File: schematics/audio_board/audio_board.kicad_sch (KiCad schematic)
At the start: 42 parts, among them J1 servo ctrl, J2 Speaker, J3 I2S, Q1 PMOS, Q2 NPN, U1 TPS613222ADBV, U2 MAX98357A, U3 TPS613222ADBV, U4 TPS613222ADBV, U8 MCP73812

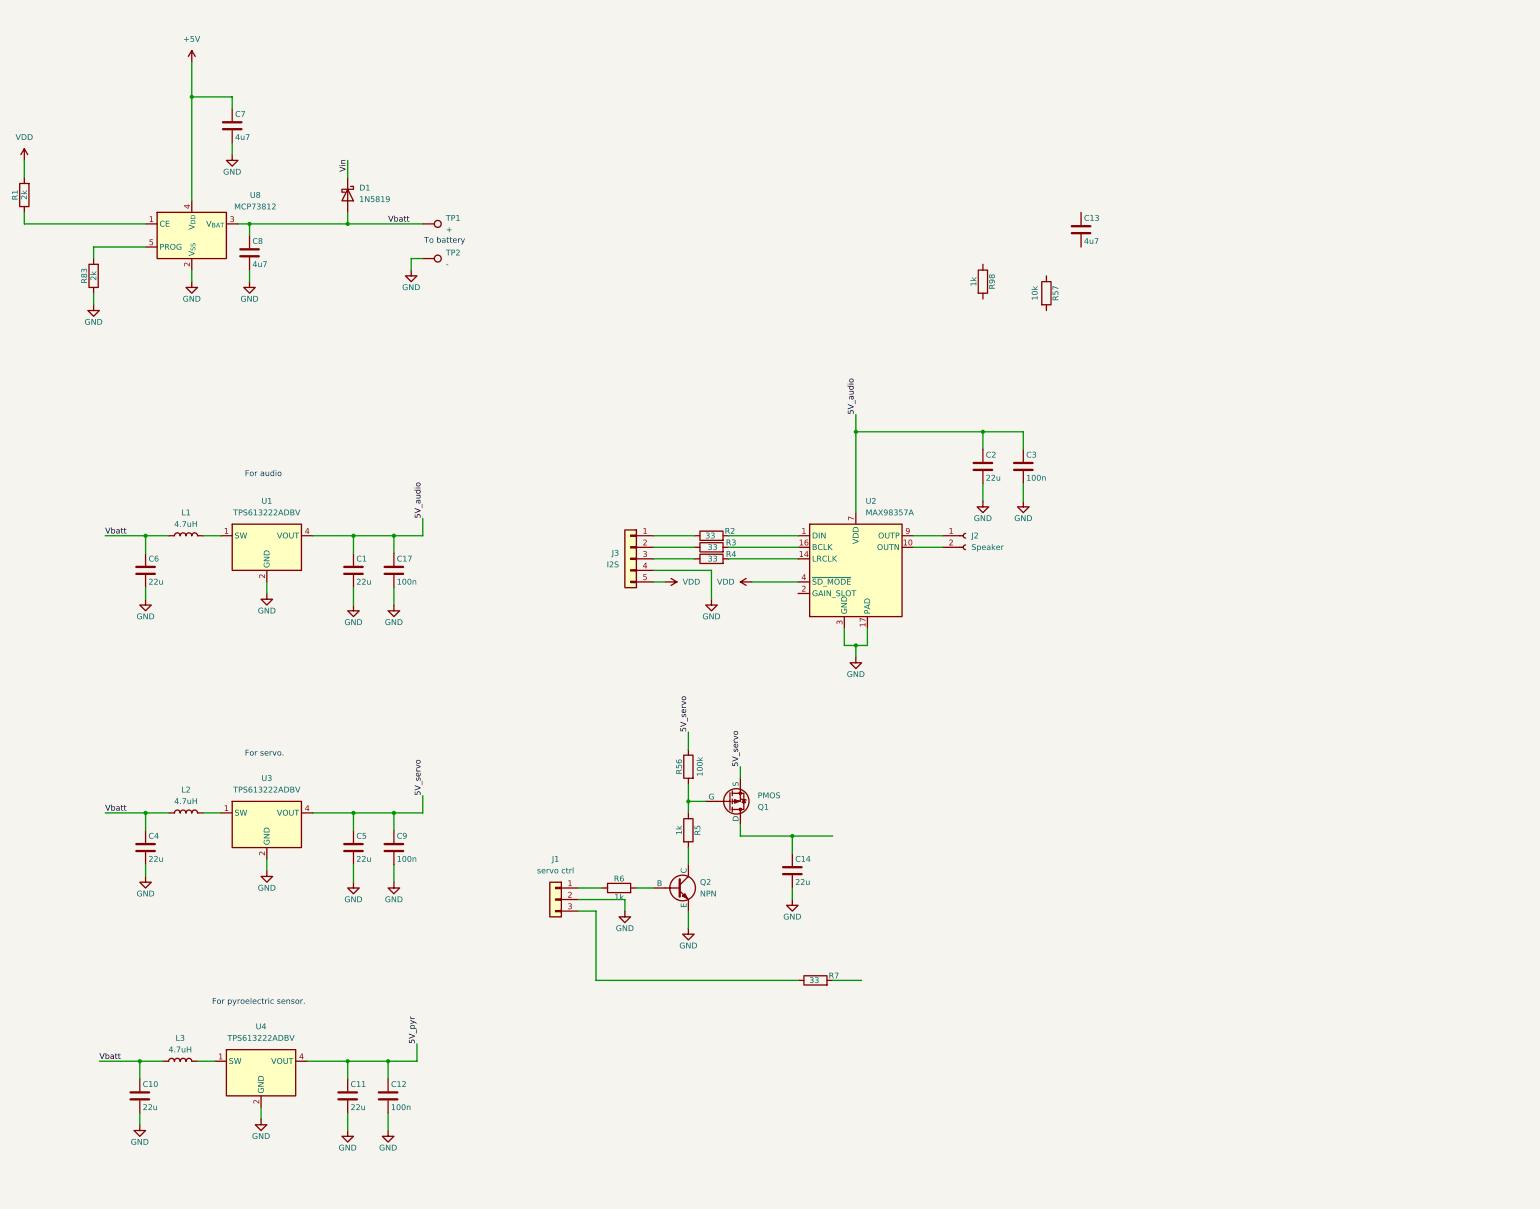
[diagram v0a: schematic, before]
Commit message: I think, the schematic is done.
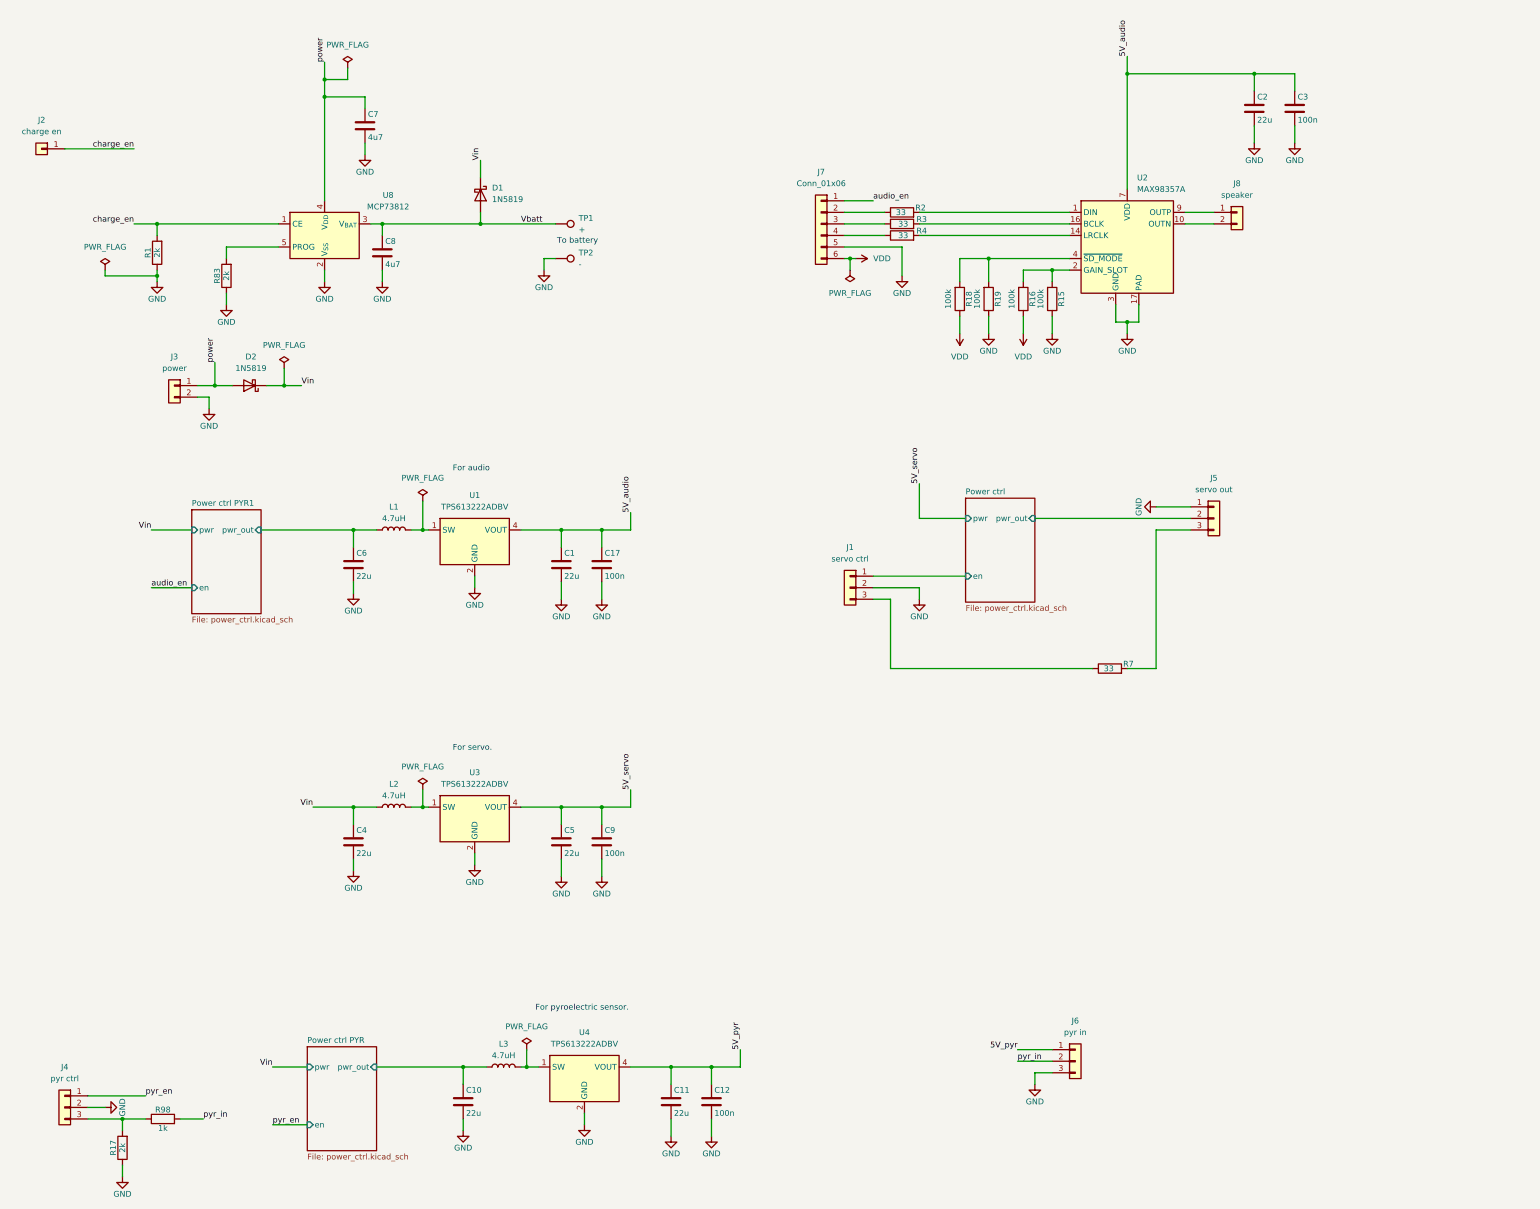
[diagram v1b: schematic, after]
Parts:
- removed C13: 4u7, Capacitor_SMD:C_0603_1608Metric, symbol Device:C
- removed C14: 22u, Capacitor_SMD:C_0603_1608Metric, symbol Device:C
- removed J2: Speaker, symbol Connector:Conn_01x02_Socket
- removed J3: I2S, symbol Connector_Generic:Conn_01x05
- removed Q1: PMOS, symbol Simulation_SPICE:PMOS
- removed Q2: NPN, symbol Simulation_SPICE:NPN
- removed R5, R6: 1k, Capacitor_SMD:C_0603_1608Metric, symbol Device:R
- removed R56: 100k, Resistor_SMD:R_0603_1608Metric, symbol Device:R
- removed R57: 10k, Capacitor_SMD:C_0603_1608Metric, symbol Device:R
- added D2: 1N5819, Diode_THT:D_DO-41_SOD81_P7.62mm_Horizontal, symbol Device:D_Schottky
- added J2: charge en, Connector_PinSocket_2.54mm:PinSocket_1x01_P2.54mm_Vertical, symbol Connector_Generic:Conn_01x01
- added J3: power, Connector_PinSocket_2.54mm:PinSocket_1x02_P2.54mm_Vertical, symbol Connector_Generic:Conn_01x02
- added J4: pyr ctrl, Connector_PinSocket_2.54mm:PinSocket_1x03_P2.54mm_Vertical, symbol Connector_Generic:Conn_01x03
- added J5: servo out, Connector_PinSocket_2.54mm:PinSocket_1x03_P2.54mm_Vertical, symbol Connector_Generic:Conn_01x03
- added J6: pyr in, Connector_PinSocket_2.54mm:PinSocket_1x03_P2.54mm_Vertical, symbol Connector_Generic:Conn_01x03
- added J7: Conn_01x06, Connector_PinSocket_2.54mm:PinSocket_1x06_P2.54mm_Vertical, symbol Connector_Generic:Conn_01x06
- added J8: speaker, Connector_PinSocket_2.54mm:PinSocket_1x02_P2.54mm_Vertical, symbol Connector_Generic:Conn_01x02
- added R15, R16, R18, R19: 100k, Resistor_SMD:R_0603_1608Metric, symbol Device:R
- added R17: 2k, Capacitor_SMD:C_0603_1608Metric, symbol Device:R
- J1: footprint (none) -> Connector_PinSocket_2.54mm:PinSocket_1x03_P2.54mm_Vertical
- R2, R3, R4, R7: footprint (none) -> Resistor_SMD:R_0201_0603Metric_Pad0.64x0.40mm_HandSolder
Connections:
- net 5V_pyr: now also J6.1 (Pin_1)
- net GND: now also R1.1, J3.2 (Pin_2), J4.2 (Pin_2), J5.1 (Pin_1), J6.3 (Pin_3), J7.5 (Pin_5), R15.1, R17.1, R19.1
- net VDD: now also J7.6 (Pin_6), R16.1, R18.1; no longer R1.2, U2.4 (~{SD_MODE})
- net Vbatt: no longer C10.1, C4.1, C6.1, L1.1, L2.1, L3.1
- net Vin: now also C4.1, L2.1, D2.1 (K)
- net Power ctrl/en: now reaches J1.1 (Pin_1)
- net charge_en: now reaches U8.1 (CE)
- net charge_en: now also R1.2, J2.1 (Pin_1); no longer R1.1
- net at R7.2: now also J5.3 (Pin_3)
- net at R2.1: now also J7.2 (Pin_2)
- net at R3.1: now also J7.3 (Pin_3)
- net at R4.1: now also J7.4 (Pin_4)
- net at U2.10 (OUTN): now also J8.2 (Pin_2)
- net at U2.2 (GAIN_SLOT): now also R15.2, R16.2
- net at U2.9 (OUTP): now also J8.1 (Pin_1)
- net at R98.1: now also J4.3 (Pin_3), R17.2
- net pyr_in: now reaches R98.2
- net pyr_in: now also J6.2 (Pin_2)
- net +5V renamed power
- net power: now also D2.2 (A), J3.1 (Pin_1)
- new net: R18.2, R19.2, U2.4 (~{SD_MODE})
- new net Power ctrl PYR/pwr_out: C10.1, L3.1
- new net Power ctrl PYR1/pwr_out: C6.1, L1.1
- new net Power ctrl/pwr_out: J5.2 (Pin_2)
- new net audio_en: J7.1 (Pin_1)
- new net pyr_en: J4.1 (Pin_1)
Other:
- added sheet Power ctrl (power_ctrl.kicad_sch)
- added sheet Power ctrl PYR (power_ctrl.kicad_sch)
- added sheet Power ctrl PYR1 (power_ctrl.kicad_sch)
- moved on the sheet: C1, C10, C11, C12, C17, C2, C3, C4, C5, C6, C7, C8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

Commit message: Placing footprints.
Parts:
- C1, C10, C11, C12, C17, C2, C3, C4, C5, C6, C7, C8, C9, R17, R83, R98: footprint Capacitor_SMD:C_0603_1608Metric -> Capacitor_SMD:C_0603_1608Metric_Pad1.08x0.95mm_HandSolder
- R1: footprint Capacitor_SMD:C_0603_1608Metric -> Resistor_SMD:R_0603_1608Metric_Pad0.98x0.95mm_HandSolder
- R15, R16, R18, R19: footprint Resistor_SMD:R_0603_1608Metric -> Resistor_SMD:R_0603_1608Metric_Pad0.98x0.95mm_HandSolder
- R2, R3, R4, R7: footprint Resistor_SMD:R_0201_0603Metric_Pad0.64x0.40mm_HandSolder -> Resistor_SMD:R_0603_1608Metric_Pad0.98x0.95mm_HandSolder
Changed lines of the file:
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@@
 			)
 		)
-		(property "Footprint" "Resistor_SMD:R_0603_1608Metric"
+		(property "Footprint" "Resistor_SMD:R_0603_1608Metric_Pad0.98x0.95mm_HandSolder"
 			(at 230.632 74.93 90)
 			(effects
@@
 			)
 		)
-		(property "Footprint" "Capacitor_SMD:C_0603_1608Metric"
+		(property "Footprint" "Capacitor_SMD:C_0603_1608Metric_Pad1.08x0.95mm_HandSolder"
 			(at 139.3952 198.12 0)
 			(effects
@@
 			)
 		)
-		(property "Footprint" "Capacitor_SMD:C_0603_1608Metric"
+		(property "Footprint" "Capacitor_SMD:C_0603_1608Metric_Pad1.08x0.95mm_HandSolder"
 			(at 172.4152 255.27 0)
 			(effects
@@
 			)
 		)
-		(property "Footprint" "Capacitor_SMD:C_0603_1608Metric"
+		(property "Footprint" "Capacitor_SMD:C_0603_1608Metric_Pad1.08x0.95mm_HandSolder"
 			(at 139.3952 137.16 0)
 			(effects
@@
 			)
 		)
-		(property "Footprint" "Capacitor_SMD:C_0603_1608Metric"
+		(property "Footprint" "Capacitor_SMD:C_0603_1608Metric_Pad1.08x0.95mm_HandSolder"
 			(at 100.0252 68.58 0)
 			(effects
@@
 			)
 		)
-		(property "Footprint" "Capacitor_SMD:C_0603_1608Metric"
+		(property "Footprint" "Capacitor_SMD:C_0603_1608Metric_Pad1.08x0.95mm_HandSolder"
 			(at 117.8052 255.27 0)
 			(effects
@@
 			)
 		)
-		(property "Footprint" "Resistor_SMD:R_0201_0603Metric_Pad0.64x0.40mm_HandSolder"
+		(property "Footprint" "Resistor_SMD:R_0603_1608Metric_Pad0.98x0.95mm_HandSolder"
 			(at 259.08 157.988 90)
 			(effects
@@
 			)
 		)
-		(property "Footprint" "Resistor_SMD:R_0603_1608Metric"
+		(property "Footprint" "Resistor_SMD:R_0603_1608Metric_Pad0.98x0.95mm_HandSolder"
 			(at 238.252 74.93 90)
 			(effects
@@
 			)
 		)
-		(property "Footprint" "Capacitor_SMD:C_0603_1608Metric"
+		(property "Footprint" "Capacitor_SMD:C_0603_1608Metric_Pad1.08x0.95mm_HandSolder"
 			(at 93.6752 137.16 0)
 			(effects
@@
 			)
 		)
-		(property "Footprint" "Capacitor_SMD:C_0603_1608Metric"
+		(property "Footprint" "Capacitor_SMD:C_0603_1608Metric_Pad1.08x0.95mm_HandSolder"
 			(at 148.2852 198.12 0)
 			(effects
@@
 			)
 		)
-		(property "Footprint" "Capacitor_SMD:C_0603_1608Metric"
+		(property "Footprint" "Capacitor_SMD:C_0603_1608Metric_Pad1.08x0.95mm_HandSolder"
 			(at 163.5252 255.27 0)
 			(effects
@@
 			)
 		)
-		(property "Footprint" "Resistor_SMD:R_0201_0603Metric_Pad0.64x0.40mm_HandSolder"
+		(property "Footprint" "Resistor_SMD:R_0603_1608Metric_Pad0.98x0.95mm_HandSolder"
 			(at 213.36 60.198 90)
 			(effects
@@
 			)
 		)
-		(property "Footprint" "Capacitor_SMD:C_0603_1608Metric"
+		(property "Footprint" "Capacitor_SMD:C_0603_1608Metric_Pad1.08x0.95mm_HandSolder"
 			(at 93.6752 198.12 0)
 			(effects
@@
 			)
 		)
-		(property "Footprint" "Capacitor_SMD:C_0603_1608Metric"
+		(property "Footprint" "Capacitor_SMD:C_0603_1608Metric_Pad1.08x0.95mm_HandSolder"
 			(at 300.6852 36.83 0)
 			(effects
@@
 			)
 		)
-		(property "Footprint" "Capacitor_SMD:C_0603_1608Metric"
+		(property "Footprint" "Capacitor_SMD:C_0603_1608Metric_Pad1.08x0.95mm_HandSolder"
 			(at 50.8 257.048 90)
 			(effects
@@
 			)
 		)
-		(property "Footprint" "Capacitor_SMD:C_0603_1608Metric"
+		(property "Footprint" "Capacitor_SMD:C_0603_1608Metric_Pad1.08x0.95mm_HandSolder"
 			(at 43.688 261.62 90)
 			(effects
@@
 			)
 		)
-		(property "Footprint" "Resistor_SMD:R_0201_0603Metric_Pad0.64x0.40mm_HandSolder"
+		(property "Footprint" "Resistor_SMD:R_0603_1608Metric_Pad0.98x0.95mm_HandSolder"
 			(at 213.36 62.738 90)
 			(effects
@@
 			)
 		)
-		(property "Footprint" "Capacitor_SMD:C_0603_1608Metric"
+		(property "Footprint" "Capacitor_SMD:C_0603_1608Metric_Pad1.08x0.95mm_HandSolder"
 			(at 66.548 69.85 90)
 			(effects
@@
 			)
 		)
-		(property "Footprint" "Capacitor_SMD:C_0603_1608Metric"
+		(property "Footprint" "Capacitor_SMD:C_0603_1608Metric_Pad1.08x0.95mm_HandSolder"
 			(at 148.2852 137.16 0)
 			(effects
@@
 			)
 		)
-		(property "Footprint" "Capacitor_SMD:C_0603_1608Metric"
+		(property "Footprint" "Capacitor_SMD:C_0603_1608Metric_Pad1.08x0.95mm_HandSolder"
 			(at 291.7952 36.83 0)
 			(effects
@@
 			)
 		)
-		(property "Footprint" "Capacitor_SMD:C_0603_1608Metric"
+		(property "Footprint" "Resistor_SMD:R_0603_1608Metric_Pad0.98x0.95mm_HandSolder"
 			(at 51.308 64.77 90)
 			(effects
@@
 			)
 		)
-		(property "Footprint" "Capacitor_SMD:C_0603_1608Metric"
+		(property "Footprint" "Capacitor_SMD:C_0603_1608Metric_Pad1.08x0.95mm_HandSolder"
 			(at 96.2152 40.64 0)
 			(effects
@@
 			)
 		)
-		(property "Footprint" "Resistor_SMD:R_0603_1608Metric"
+		(property "Footprint" "Resistor_SMD:R_0603_1608Metric_Pad0.98x0.95mm_HandSolder"
 			(at 244.602 74.93 90)
 			(effects
@@
 			)
 		)
-		(property "Footprint" "Resistor_SMD:R_0201_0603Metric_Pad0.64x0.40mm_HandSolder"
+		(property "Footprint" "Resistor_SMD:R_0603_1608Metric_Pad0.98x0.95mm_HandSolder"
 			(at 213.36 57.658 90)
 			(effects
@@
 			)
 		)
-		(property "Footprint" "Resistor_SMD:R_0603_1608Metric"
+		(property "Footprint" "Resistor_SMD:R_0603_1608Metric_Pad0.98x0.95mm_HandSolder"
 			(at 224.282 74.93 90)
 			(effects

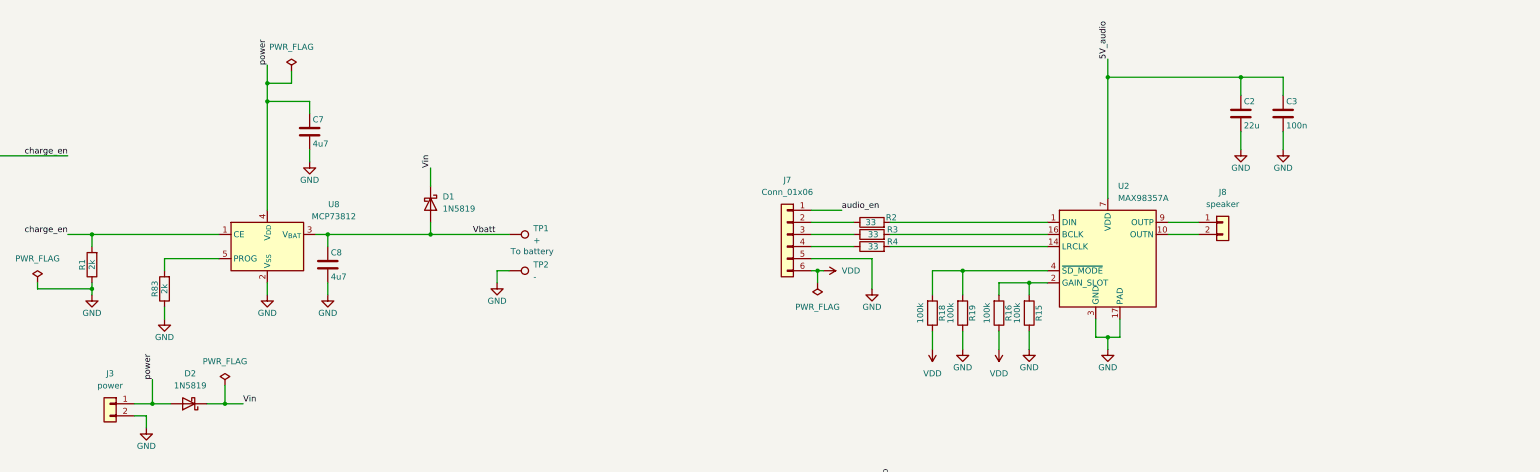
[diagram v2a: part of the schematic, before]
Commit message: a
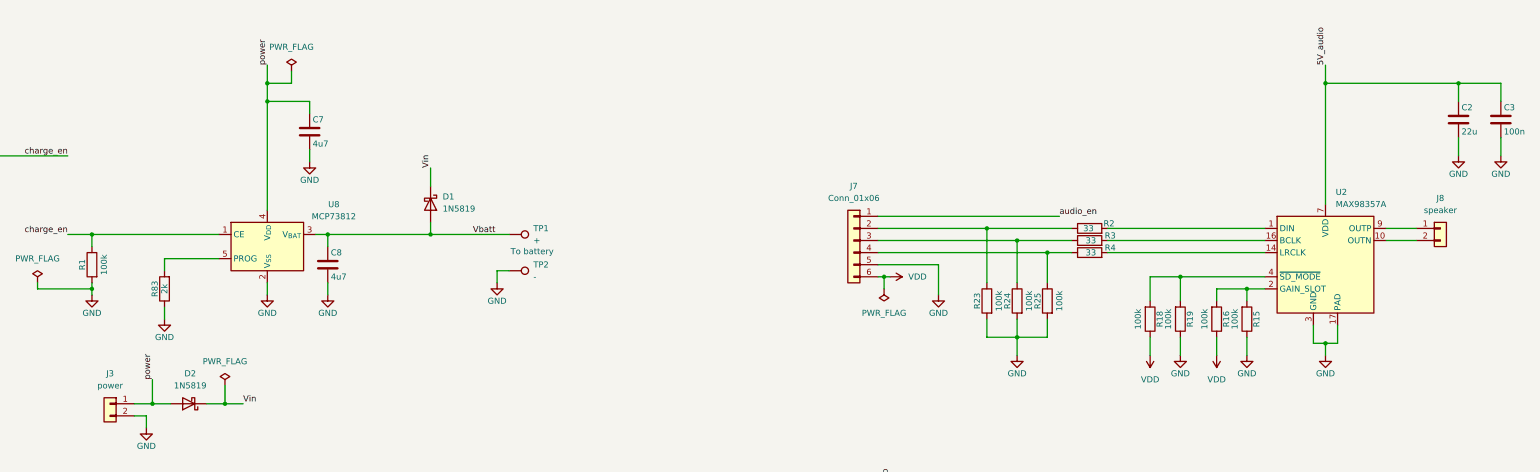
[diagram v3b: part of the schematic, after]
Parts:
- added R23, R24, R25: 100k, Resistor_SMD:R_0603_1608Metric_Pad0.98x0.95mm_HandSolder, symbol Device:R
- R1: value 2k -> 100k; URL https://www.digikey.com/en/products/detail/yageo/AC0603JR-0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 -> (none)
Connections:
- net GND: now also R1.2, R23.2, R24.2, R25.2; no longer R1.1
- net charge_en: now also R1.1; no longer R1.2
- net at J7.3 (Pin_3), R3.1: now also R24.1
- net at J7.4 (Pin_4), R4.1: now also R25.1
- net at J7.2 (Pin_2), R2.1: now also R23.1
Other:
- moved on the sheet: C2, C3, J7, J8, R15, R16, R18, R19, R2, R3, R4, U2
